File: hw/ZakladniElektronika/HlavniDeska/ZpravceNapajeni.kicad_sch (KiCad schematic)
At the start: 0 parts

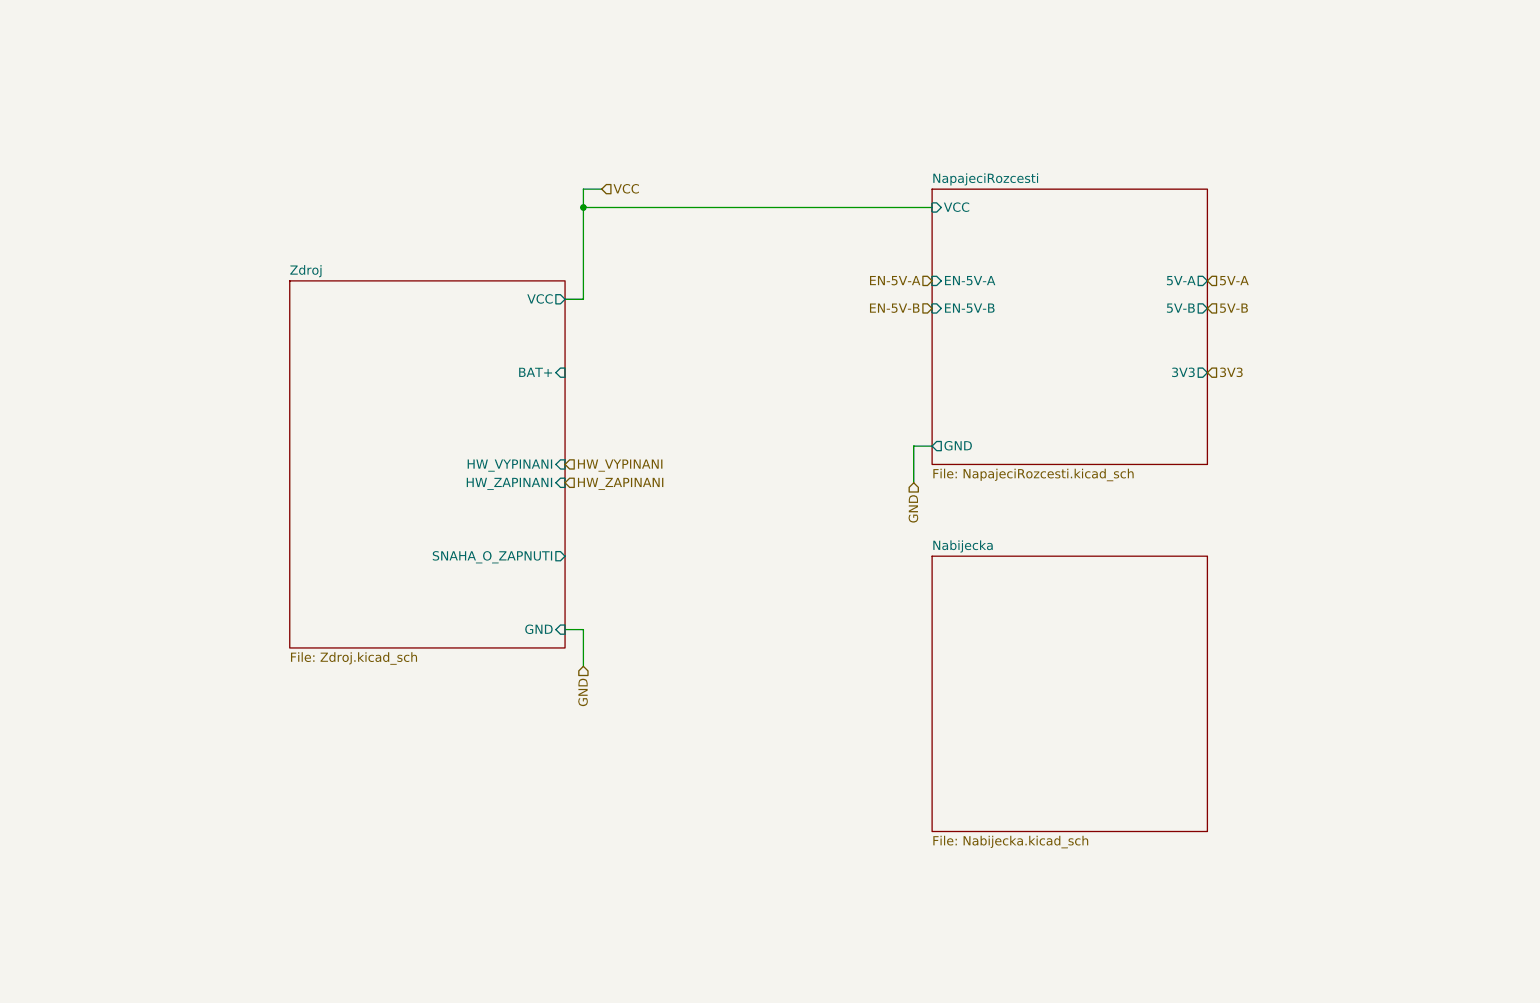
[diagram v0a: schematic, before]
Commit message: WIP
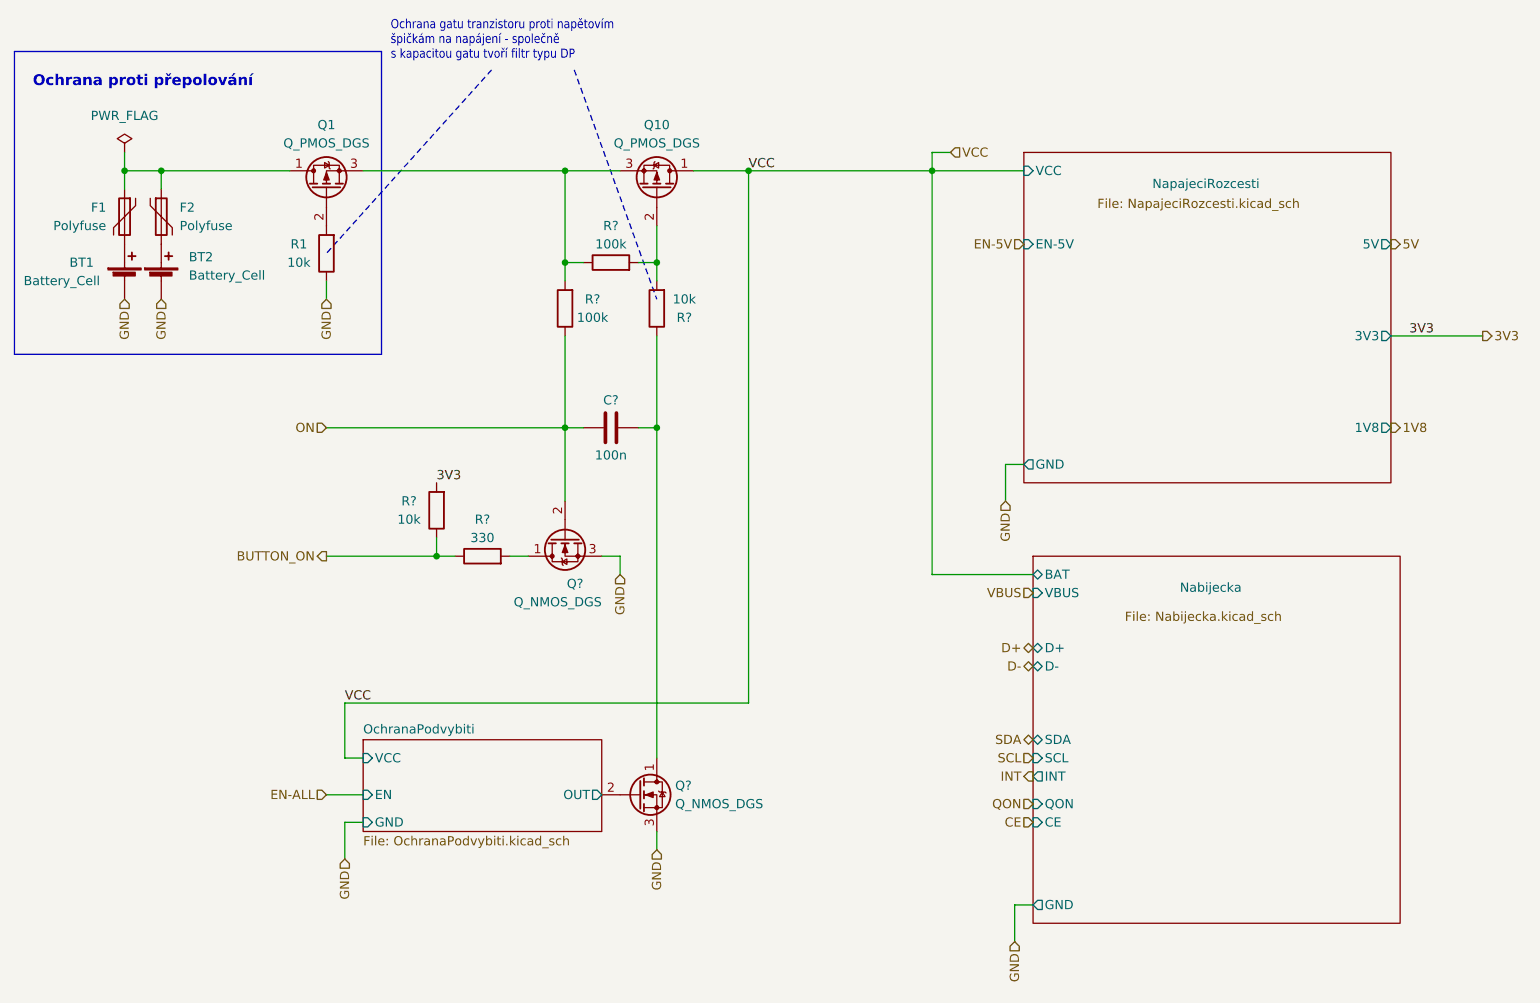
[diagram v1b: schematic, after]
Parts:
- added BT1, BT2: Battery_Cell, symbol Device:Battery_Cell
- added C?: 100n, Capacitor_SMD:C_0402_1005Metric, symbol Device:C
- added F1, F2: Polyfuse, Inductor_SMD:L_1206_3216Metric, symbol Device:Polyfuse
- added Q1, Q10: Q_PMOS_DGS, RBCX:JMSL0302AU, symbol Device:Q_PMOS_DGS
- added Q? (x2): Q_NMOS_DGS, Package_TO_SOT_SMD:SOT-723, symbol Device:Q_NMOS_DGS
- added R1, R? (x2): 10k, Capacitor_SMD:C_0201_0603Metric, symbol Device:R
- added R? (x2): 100k, Capacitor_SMD:C_0201_0603Metric, symbol Device:R
- added R?: 330, Capacitor_SMD:C_0201_0603Metric, symbol Device:R
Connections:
- net 3V3: now also R?.2
- net GND: now also BT1.2 (-), BT2.2 (-), Q?.3 (S), Q?.3 (S), R1.1
- net VCC: now also Q10.1 (D)
- new net: BT2.1 (+), F2.2
- new net: Q1.2 (G), R1.2
- new net: Q1.3 (S), Q10.3 (S), R?.1, R?.2
- new net: F1.1, F2.1, Q1.1 (D)
- new net: C?.2, Q?.1 (D), R?.1
- new net: Q10.2 (G), R?.2, R?.2
- new net: Q?.1 (D), R?.2
- new net: BT1.1 (+), F1.2
- new net BUTTON_ON: R?.1, R?.1
- new net ON: C?.1, Q?.2 (G), R?.1
- new net OchranaPodvybiti/OUT: Q?.2 (G)
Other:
- removed sheet Zdroj
- added sheet OchranaPodvybiti (OchranaPodvybiti.kicad_sch)
- sheet Nabijecka ports: added BAT, CE, D+, D-, GND, INT, QON, SCL, SDA, VBUS; removed none
- sheet NapajeciRozcesti ports: added 1V8, 5V, EN-5V; removed 5V-A, 5V-B, EN-5V-A, EN-5V-B
- note added: "Ochrana gatu tranzistoru proti napětovím špičkám na napájení - společně s kapacitou gatu tvoří filtr typu DP"
- note added: "Ochrana proti přepolování"
